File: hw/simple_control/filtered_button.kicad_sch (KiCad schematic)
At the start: 4 parts, among them SW602 SW_Push

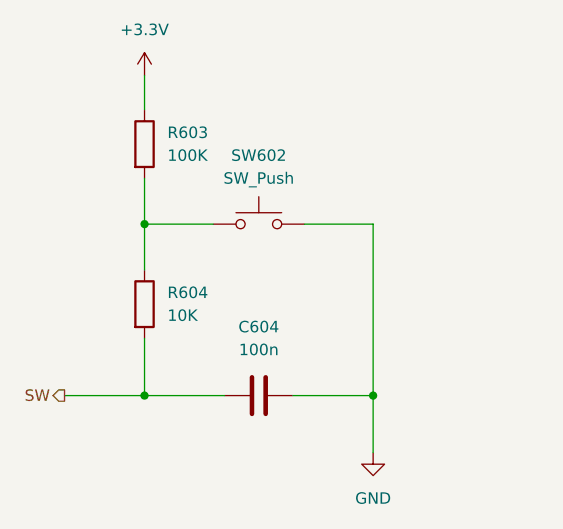
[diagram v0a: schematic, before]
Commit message: chore(hw): add buttons layout
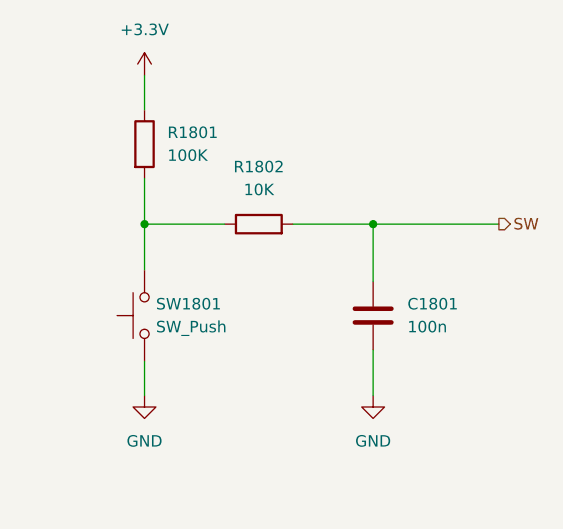
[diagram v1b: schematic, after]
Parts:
- renumbered C604 to C1801, R603 to R1801, R604 to R1802, SW602 to SW1801
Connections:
- net GND: now also C1801.1, SW1801.1; no longer C1801.2, SW1801.2
- net SW: now also C1801.2; no longer C1801.1
- net at R1801.2, R1802.1: now also SW1801.2; no longer SW1801.1
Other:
- moved on the sheet: C1801, R1802, SW1801
